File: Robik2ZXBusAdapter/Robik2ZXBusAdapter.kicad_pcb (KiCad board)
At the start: 2 copper layers, 55.9 x 94 mm, 8 parts, among them Q1 BC558, Q2 BC558, U1 RobikBUS

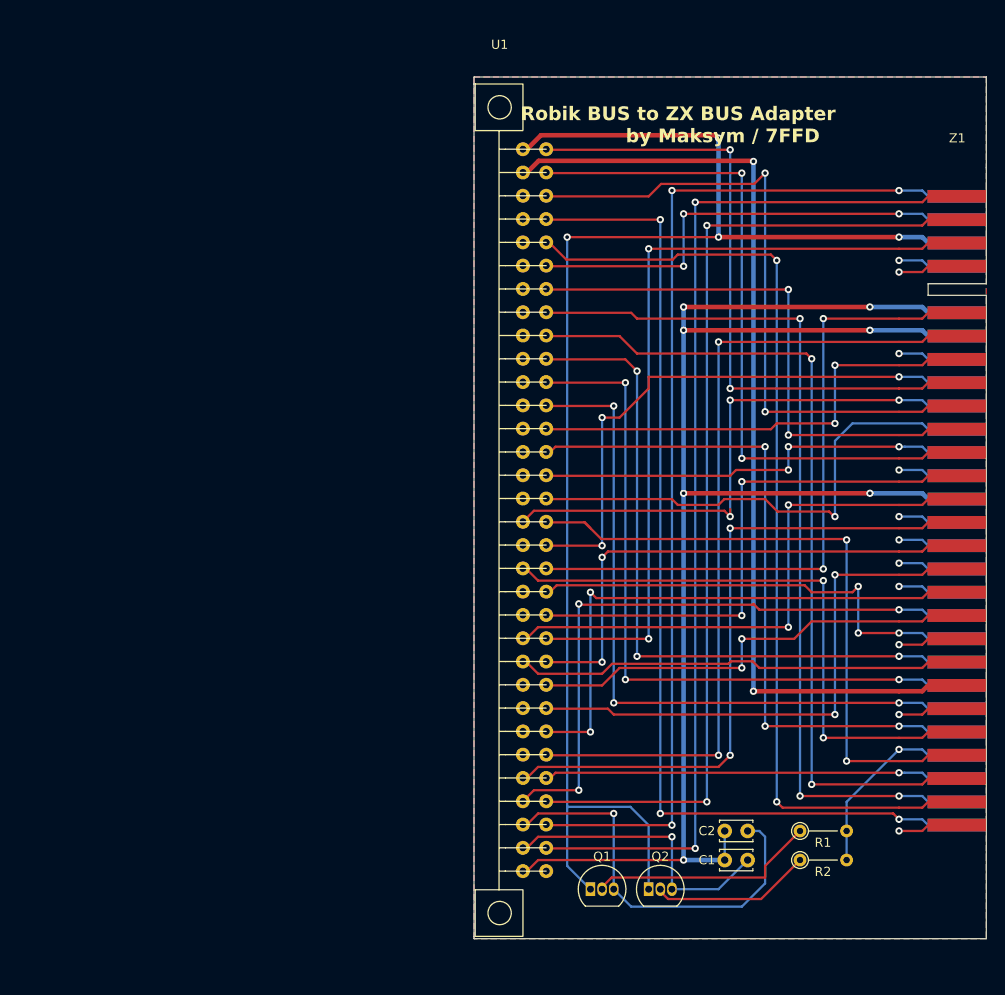
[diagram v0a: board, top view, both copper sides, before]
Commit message: fixed issues
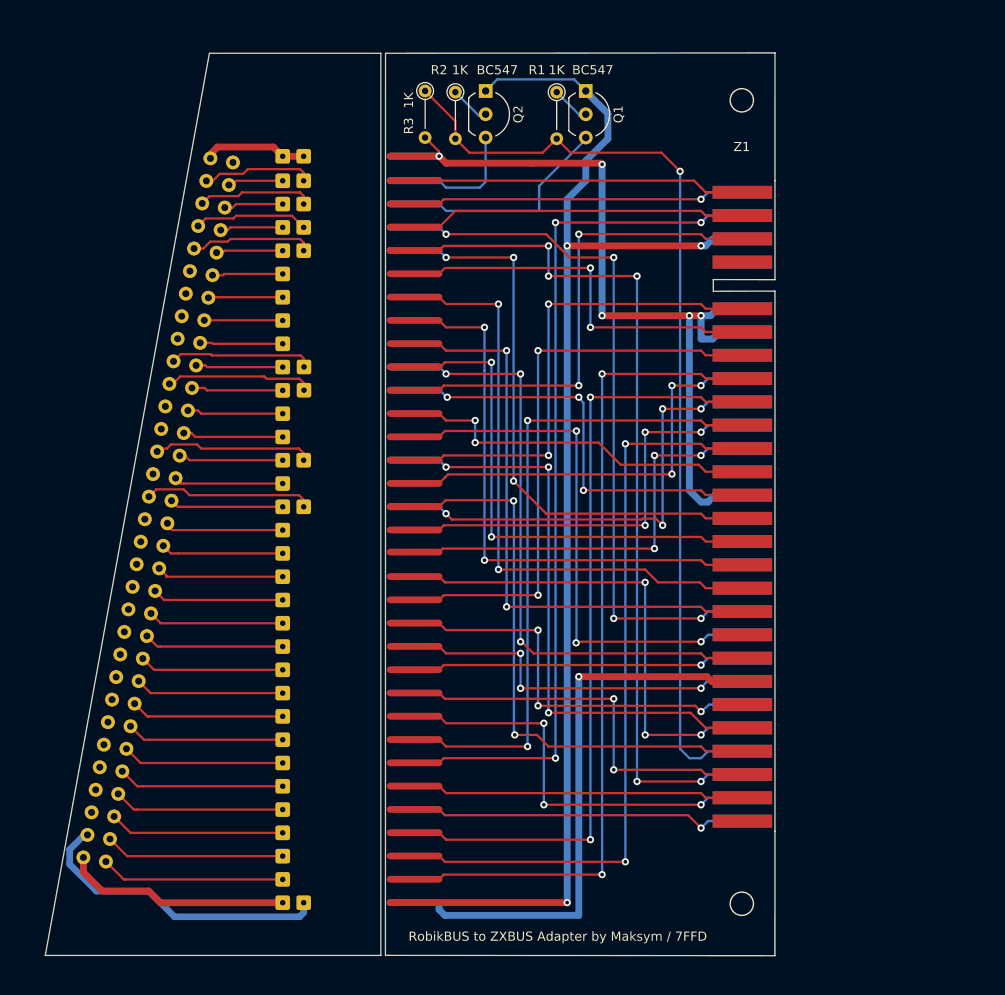
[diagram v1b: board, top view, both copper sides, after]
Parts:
- removed C1, C2: 220, Capacitor_THT:C_Disc_D3.4mm_W2.1mm_P2.50mm
- added R3: 1K, Resistor_THT:R_Axial_DIN0204_L3.6mm_D1.6mm_P5.08mm_Vertical, F.Cu at (115.3, 44.7)
- added REF**: SolderWire-0.1sqmm_1x01_D0.4mm_OD1mm, RobikBUS:SolderWire-0.1sqmm_1x01_D0.4mm_OD1mm, F.Cu at (99.8, 118.0)
- added REF**: SolderWire-0.1sqmm_1x01_D0.4mm_OD1mm, RobikBUS:SolderWire-0.1sqmm_1x01_D0.4mm_OD1mm, F.Cu at (99.8, 107.8)
- added REF**: SolderWire-0.1sqmm_1x01_D0.4mm_OD1mm, RobikBUS:SolderWire-0.1sqmm_1x01_D0.4mm_OD1mm, F.Cu at (102.1, 77.3)
- added REF**: SolderWire-0.1sqmm_1x01_D0.4mm_OD1mm, RobikBUS:SolderWire-0.1sqmm_1x01_D0.4mm_OD1mm, F.Cu at (99.8, 82.4)
- added REF**: SolderWire-0.1sqmm_1x01_D0.4mm_OD1mm, RobikBUS:SolderWire-0.1sqmm_1x01_D0.4mm_OD1mm, F.Cu at (99.8, 133.2)
- added REF**: SolderWire-0.1sqmm_1x01_D0.4mm_OD1mm, RobikBUS:SolderWire-0.1sqmm_1x01_D0.4mm_OD1mm, F.Cu at (99.8, 105.3)
- added REF**: SolderWire-0.1sqmm_1x01_D0.4mm_OD1mm, RobikBUS:SolderWire-0.1sqmm_1x01_D0.4mm_OD1mm, F.Cu at (99.8, 95.1)
- added REF**: SolderWire-0.1sqmm_1x01_D0.4mm_OD1mm, RobikBUS:SolderWire-0.1sqmm_1x01_D0.4mm_OD1mm, F.Cu at (99.8, 51.8)
- added REF**: SolderWire-0.1sqmm_1x01_D0.4mm_OD1mm, RobikBUS:SolderWire-0.1sqmm_1x01_D0.4mm_OD1mm, F.Cu at (99.8, 59.6)
- added REF**: SolderWire-0.1sqmm_1x01_D0.4mm_OD1mm, RobikBUS:SolderWire-0.1sqmm_1x01_D0.4mm_OD1mm, F.Cu at (102.1, 54.5)
- added REF**: SolderWire-0.1sqmm_1x01_D0.4mm_OD1mm, RobikBUS:SolderWire-0.1sqmm_1x01_D0.4mm_OD1mm, F.Cu at (102.1, 62.1)
- added REF**: SolderWire-0.1sqmm_1x01_D0.4mm_OD1mm, RobikBUS:SolderWire-0.1sqmm_1x01_D0.4mm_OD1mm, F.Cu at (99.8, 92.6)
- added REF**: SolderWire-0.1sqmm_1x01_D0.4mm_OD1mm, RobikBUS:SolderWire-0.1sqmm_1x01_D0.4mm_OD1mm, F.Cu at (99.8, 128.2)
- added REF**: SolderWire-0.1sqmm_1x01_D0.4mm_OD1mm, RobikBUS:SolderWire-0.1sqmm_1x01_D0.4mm_OD1mm, F.Cu at (99.8, 85.0)
- added REF**: SolderWire-0.1sqmm_1x01_D0.4mm_OD1mm, RobikBUS:SolderWire-0.1sqmm_1x01_D0.4mm_OD1mm, F.Cu at (99.8, 69.7)
- added REF**: SolderWire-0.1sqmm_1x01_D0.4mm_OD1mm, RobikBUS:SolderWire-0.1sqmm_1x01_D0.4mm_OD1mm, F.Cu at (99.8, 79.9)
- added REF**: SolderWire-0.1sqmm_1x01_D0.4mm_OD1mm, RobikBUS:SolderWire-0.1sqmm_1x01_D0.4mm_OD1mm, F.Cu at (99.8, 120.5)
- added REF**: SolderWire-0.1sqmm_1x01_D0.4mm_OD1mm, RobikBUS:SolderWire-0.1sqmm_1x01_D0.4mm_OD1mm, F.Cu at (102.1, 85.0)
- added REF**: SolderWire-0.1sqmm_1x01_D0.4mm_OD1mm, RobikBUS:SolderWire-0.1sqmm_1x01_D0.4mm_OD1mm, F.Cu at (102.1, 51.8)
- added REF**: SolderWire-0.1sqmm_1x01_D0.4mm_OD1mm, RobikBUS:SolderWire-0.1sqmm_1x01_D0.4mm_OD1mm, F.Cu at (99.8, 67.2)
- added REF**: SolderWire-0.1sqmm_1x01_D0.4mm_OD1mm, RobikBUS:SolderWire-0.1sqmm_1x01_D0.4mm_OD1mm, F.Cu at (99.8, 110.4)
- added REF**: SolderWire-0.1sqmm_1x01_D0.4mm_OD1mm, RobikBUS:SolderWire-0.1sqmm_1x01_D0.4mm_OD1mm, F.Cu at (99.8, 97.7)
- added REF**: SolderWire-0.1sqmm_1x01_D0.4mm_OD1mm, RobikBUS:SolderWire-0.1sqmm_1x01_D0.4mm_OD1mm, F.Cu at (99.8, 57.0)
- added REF**: SolderWire-0.1sqmm_1x01_D0.4mm_OD1mm, RobikBUS:SolderWire-0.1sqmm_1x01_D0.4mm_OD1mm, F.Cu at (99.8, 100.2)
- added REF**: SolderWire-0.1sqmm_1x01_D0.4mm_OD1mm, RobikBUS:SolderWire-0.1sqmm_1x01_D0.4mm_OD1mm, F.Cu at (99.8, 72.3)
- added REF**: SolderWire-0.1sqmm_1x01_D0.4mm_OD1mm, RobikBUS:SolderWire-0.1sqmm_1x01_D0.4mm_OD1mm, F.Cu at (99.8, 64.7)
- added REF**: SolderWire-0.1sqmm_1x01_D0.4mm_OD1mm, RobikBUS:SolderWire-0.1sqmm_1x01_D0.4mm_OD1mm, F.Cu at (99.8, 77.4)
- added REF**: SolderWire-0.1sqmm_1x01_D0.4mm_OD1mm, RobikBUS:SolderWire-0.1sqmm_1x01_D0.4mm_OD1mm, F.Cu at (99.8, 90.1)
- added REF**: SolderWire-0.1sqmm_1x01_D0.4mm_OD1mm, RobikBUS:SolderWire-0.1sqmm_1x01_D0.4mm_OD1mm, F.Cu at (99.8, 123.1)
- added REF**: SolderWire-0.1sqmm_1x01_D0.4mm_OD1mm, RobikBUS:SolderWire-0.1sqmm_1x01_D0.4mm_OD1mm, F.Cu at (99.8, 112.9)
- added REF**: SolderWire-0.1sqmm_1x01_D0.4mm_OD1mm, RobikBUS:SolderWire-0.1sqmm_1x01_D0.4mm_OD1mm, F.Cu at (102.1, 59.6)
- added REF**: SolderWire-0.1sqmm_1x01_D0.4mm_OD1mm, RobikBUS:SolderWire-0.1sqmm_1x01_D0.4mm_OD1mm, F.Cu at (99.8, 74.8)
- added REF**: SolderWire-0.1sqmm_1x01_D0.4mm_OD1mm, RobikBUS:SolderWire-0.1sqmm_1x01_D0.4mm_OD1mm, F.Cu at (99.8, 130.7)
- added REF**: SolderWire-0.1sqmm_1x01_D0.4mm_OD1mm, RobikBUS:SolderWire-0.1sqmm_1x01_D0.4mm_OD1mm, F.Cu at (102.1, 74.8)
- added REF**: SolderWire-0.1sqmm_1x01_D0.4mm_OD1mm, RobikBUS:SolderWire-0.1sqmm_1x01_D0.4mm_OD1mm, F.Cu at (102.1, 90.1)
- added REF**: SolderWire-0.1sqmm_1x01_D0.4mm_OD1mm, RobikBUS:SolderWire-0.1sqmm_1x01_D0.4mm_OD1mm, F.Cu at (99.8, 87.5)
- added REF**: SolderWire-0.1sqmm_1x01_D0.4mm_OD1mm, RobikBUS:SolderWire-0.1sqmm_1x01_D0.4mm_OD1mm, F.Cu at (99.8, 54.5)
- added REF**: SolderWire-0.1sqmm_1x01_D0.4mm_OD1mm, RobikBUS:SolderWire-0.1sqmm_1x01_D0.4mm_OD1mm, F.Cu at (102.1, 57.0)
- added REF**: SolderWire-0.1sqmm_1x01_D0.4mm_OD1mm, RobikBUS:SolderWire-0.1sqmm_1x01_D0.4mm_OD1mm, F.Cu at (102.1, 133.2)
- added REF**: SolderWire-0.1sqmm_1x01_D0.4mm_OD1mm, RobikBUS:SolderWire-0.1sqmm_1x01_D0.4mm_OD1mm, F.Cu at (99.8, 115.5)
- added REF**: SolderWire-0.1sqmm_1x01_D0.4mm_OD1mm, RobikBUS:SolderWire-0.1sqmm_1x01_D0.4mm_OD1mm, F.Cu at (99.8, 102.8)
- added REF**: SolderWire-0.1sqmm_1x01_D0.4mm_OD1mm, RobikBUS:SolderWire-0.1sqmm_1x01_D0.4mm_OD1mm, F.Cu at (99.8, 125.6)
- added REF**: SolderWire-0.1sqmm_1x01_D0.4mm_OD1mm, RobikBUS:SolderWire-0.1sqmm_1x01_D0.4mm_OD1mm, F.Cu at (99.8, 62.1)
- Q1, Q2: value BC558 -> BC547; footprint Package_TO_SOT_THT:TO-92_Inline -> Package_TO_SOT_THT:TO-92_Inline_Wide
- U1: footprint RobikBUS:RobikBUS -> RobikBUS:RobikBUS_VERT; moved to B.Cu
- moved R2 91.8 mm to (118.6, 44.8), turned to -90 degrees
- moved Q2 88.9 mm to (121.9, 44.7), turned to -90 degrees
- moved Q1 87.1 mm to (132.8, 44.7), turned to -90 degrees
- moved R1 84.8 mm to (129.7, 44.8), turned to -90 degrees
- moved U1 28.9 mm to (95.4, 46.3), turned to -100.3 degrees
- moved Z1 23.4 mm to (149.9, 48.1)
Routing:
- net //ROMCS: track 21.0 -> 104.3 mm
- net /A15: track 115.2 -> 45.0 mm, vias 2 -> 0
- net /A14: track 113.9 -> 45.4 mm, vias 3 -> 1
- net /GND: track 176.0 -> 110.6 mm, vias 7 -> 5
- net /A12: track 50.4 -> 115.1 mm
- net /A13: track 107.6 -> 46.3 mm, vias 2 -> 0
- net //BUSACK: track 45.0 -> 104.7 mm, vias 1 -> 5
- net /A11: track 109.7 -> 58.2 mm, vias 3 -> 1
- net /A10: track 105.3 -> 57.1 mm, vias 2 -> 0
- net /D6: track 70.7 -> 113.5 mm
- net /D1: track 89.8 -> 53.1 mm
- net //WAIT: track 48.6 -> 84.3 mm, vias 0 -> 3
- net /D5: track 71.8 -> 106.3 mm
- net /A9: track 97.0 -> 64.7 mm
- net /D3: track 60.6 -> 91.7 mm
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- removed copper zone on B.Cu, net /GND
- removed copper zone on F.Cu, net /GND
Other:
- board size 55.9 x 94 mm -> 79.6 x 98.5 mm
- board text added: "RobikBUS to ZXBUS Adapter by Maksym / 7FFD"
- board text removed: "Robik BUS to ZX BUS Adapter by Maksym / 7FFD"

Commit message: robik bus changes
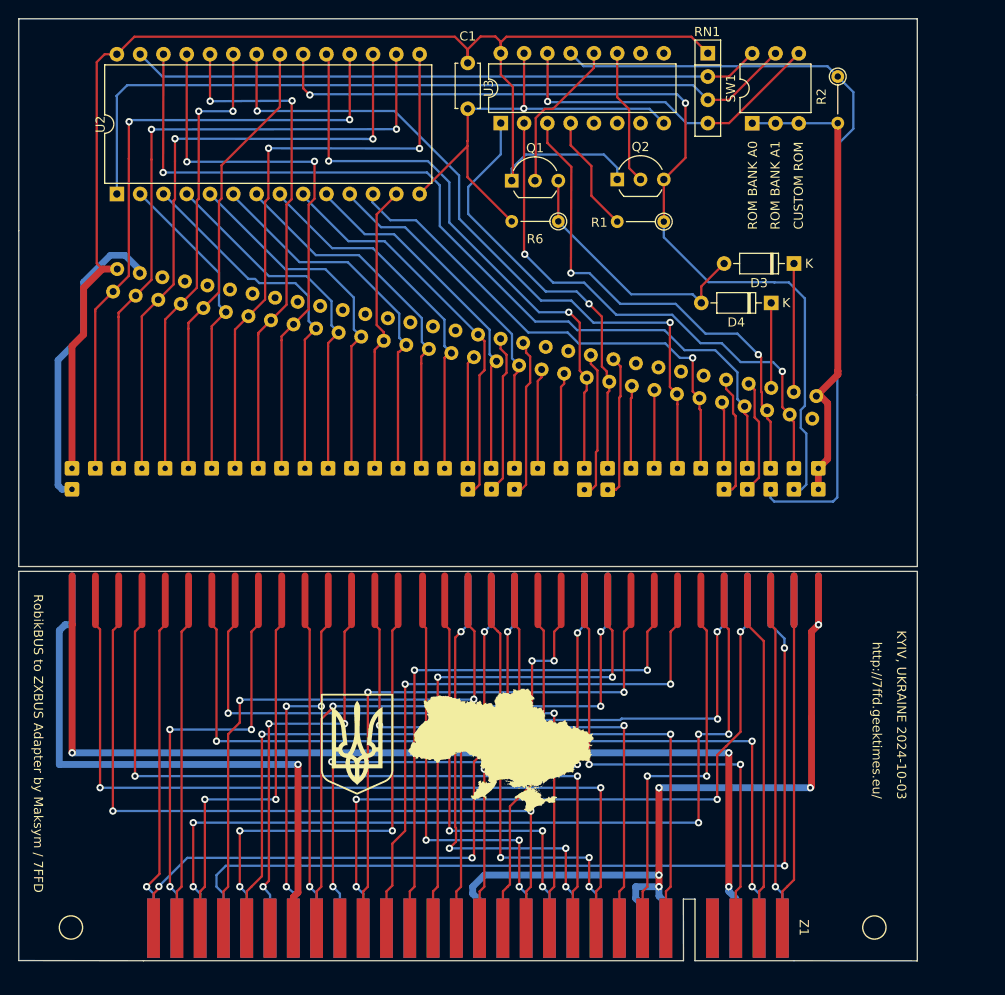
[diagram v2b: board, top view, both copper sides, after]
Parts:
- removed R3: 1K, Resistor_THT:R_Axial_DIN0204_L3.6mm_D1.6mm_P5.08mm_Vertical
- added C1: 0.1uF, Capacitor_THT:C_Disc_D4.7mm_W2.5mm_P5.00mm, F.Cu at (120.0, 41.6)
- added D3: 1N4148, Diode_THT:D_DO-35_SOD27_P7.62mm_Horizontal, F.Cu at (155.5, 63.5)
- added D4: 1N4148, Diode_THT:D_DO-35_SOD27_P7.62mm_Horizontal, F.Cu at (153.1, 67.8)
- added MAP: UA CoA 21x14mm, Symbol:UA map 21x14mm Silk, F.Cu at (124.3, 109.6)
- added R6: 1K, Resistor_THT:R_Axial_DIN0204_L3.6mm_D1.6mm_P5.08mm_Vertical, F.Cu at (129.8, 58.9)
- added REF**: SolderWire-0.1sqmm_1x01_D0.4mm_OD1mm, RobikBUS:SolderWire-0.1sqmm_1x01_D0.4mm_OD1mm, F.Cu at (122.6, 88.1)
- added RN1: 10k, Resistor_THT:R_Array_SIP4, F.Cu at (146.2, 40.6)
- added SW1: SW_DIP_x03, Package_DIP:DIP-6_W7.62mm, F.Cu at (151.0, 48.2)
- added U2: 27C512, Package_DIP:DIP-28_W15.24mm, F.Cu at (81.7, 55.9)
- added U3: 74LS139, Package_DIP:DIP-16_W7.62mm, F.Cu at (123.6, 48.2)
- added UA CoA: UA CoA 8x11mm, Symbol:UA CoA 8x11mm, F.Cu at (107.9, 109.9)
- R1, R2: value 1K -> 1k
- moved Z1 88.7 mm to (161.9, 136.0), turned to -90 degrees
- moved U1 76.9 mm to (163.8, 81.5), turned to 169.7 degrees
- moved REF** 67.6 mm to (158.2, 85.9), turned to -90 degrees
- moved REF** 66.9 mm to (158.2, 88.2), turned to -90 degrees
- moved REF** 64.0 mm to (155.5, 85.9), turned to -90 degrees
- moved REF** 63.2 mm to (155.5, 88.2), turned to -90 degrees
- moved REF** 60.5 mm to (153.0, 85.9), turned to -90 degrees
- moved REF** 59.7 mm to (153.0, 88.2), turned to -90 degrees
- moved REF** 57.1 mm to (150.5, 85.9), turned to -90 degrees
- moved REF** 56.2 mm to (150.5, 88.2), turned to -90 degrees
- moved REF** 53.7 mm to (147.9, 85.9), turned to -90 degrees
- moved REF** 52.7 mm to (147.9, 88.2), turned to -90 degrees
- moved REF** 52.7 mm to (76.8, 85.9), turned to -90 degrees
- moved REF** 51.7 mm to (76.8, 88.2), turned to -90 degrees
- moved REF** 50.3 mm to (145.4, 85.9), turned to -90 degrees
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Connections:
- Q1 pad 3: Net-(Q1-E) -> Net-(D3-A)
- R1 pad 1: Net-(Q1-B) -> Net-(Q2-E)
- R1 pad 2: //ROMCS -> Net-(U3A-O0)
- R2 pad 1: Net-(Q2-B) -> //ROMCS
- R2 pad 2: //ROMCS -> /GND
- REF** pad : Net-(Q1-E) -> //ROMCS
- U1 pad A18: unconnected-(U1-NC-PadA18) -> //KJOYCS
- U1 pad A30: Net-(Q1-E) -> Net-(D4-K)
- U1 pad A31: Net-(Q2-E) -> Net-(D3-K)
- Z1 pad A28: unconnected-(Z1-NC-PadA28) -> //KJOYCS
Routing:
- net /+5V: track 166.6 -> 263.3 mm
- net /A13: track 46.3 -> 137.5 mm, vias 0 -> 1
- net //KJOYCS: track 0.00 -> 89.5 mm, vias 0 -> 3
- net /GND: track 110.6 -> 197.8 mm, vias 5 -> 6
- net /BANK_A1: track 0.00 -> 85.8 mm
- net //ROMCS: track 104.3 -> 186.8 mm, vias 1 -> 2
- net Net-(Q2-E): track 28.5 -> 107.5 mm, vias 0 -> 2
- net //RD: track 76.7 -> 148.6 mm, vias 2 -> 4
- net /BANK_A0: track 0.00 -> 68.8 mm
- net /D7: track 65.4 -> 120.8 mm, vias 2 -> 4
- net /D4: track 104.1 -> 157.8 mm, vias 2 -> 4
- net /A15: track 45.0 -> 97.8 mm, vias 0 -> 2
- net /D6: track 113.5 -> 164.0 mm, vias 2 -> 4
- net /D5: track 106.3 -> 155.5 mm, vias 2 -> 4
- net /A14: track 45.4 -> 93.5 mm, vias 1 -> 3
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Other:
- board size 79.6 x 98.5 mm -> 98 x 102.8 mm
- board text added: "${COMMENT1}"
- board text added: "${COMMENT2} ${ISSUE_DATE}"
- board text added: "${TITLE} by ${COMPANY}"
- board text added: "CUSTOM ROM"
- board text added: "ROM BANK A0"
- board text added: "ROM BANK A1"
- board text removed: "RobikBUS to ZXBUS Adapter by Maksym / 7FFD"
